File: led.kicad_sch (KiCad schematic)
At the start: 2 parts, among them J6 Conn_01x02

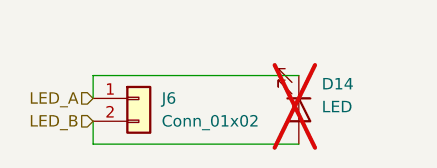
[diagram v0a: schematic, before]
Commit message: board interconnects
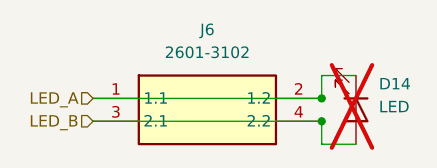
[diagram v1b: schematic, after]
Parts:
- removed J6: Conn_01x02, Connector_Wire:SolderWire-0.75sqmm_1x02_P4.8mm_D1.25mm_OD2.3mm, symbol Connector_Generic:Conn_01x02
- added J6: 2601-3102, KiCad:26013102, symbol 2601-3102:2601-3102
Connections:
- net LED_A: now also J6.1 (1.1), J6.2 (1.2)
- net LED_B: now also J6.3 (2.1), J6.4 (2.2)
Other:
- moved on the sheet: D14
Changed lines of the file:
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@@
 		(comment 3 "Bryan, Tahje")
 	)
-	(wire
-		(pts
-			(xy 171.45 106.68) (xy 148.59 106.68)
-		)
-		(stroke
-			(width 0)
-			(type default)
-		)
-	)
-	(wire
-		(pts
-			(xy 148.59 106.68) (xy 148.59 104.14)
-		)
-		(stroke
-			(width 0)
-			(type default)
-		)
-	)
-	(wire
-		(pts
-			(xy 171.45 99.06) (xy 148.59 99.06)
-		)
-		(stroke
-			(width 0)
-			(type default)
-		)
-	)
-	(wire
-		(pts
-			(xy 148.59 99.06) (xy 148.59 101.6)
+	(junction
+		(at 173.99 104.14)
+		(diameter 0)
+		(color 0 0 0 0)
+	)
+	(junction
+		(at 173.99 101.6)
+		(diameter 0)
+		(color 0 0 0 0)
+	)
+	(wire
+		(pts
+			(xy 148.59 101.6) (xy 173.99 101.6)
+		)
+		(stroke
+			(width 0)
+			(type default)
+		)
+	)
+	(wire
+		(pts
+			(xy 173.99 106.68) (xy 177.8 106.68)
+		)
+		(stroke
+			(width 0)
+			(type default)
+		)
+	)
+	(wire
+		(pts
+			(xy 173.99 104.14) (xy 173.99 106.68)
+		)
+		(stroke
+			(width 0)
+			(type default)
+		)
+	)
+	(wire
+		(pts
+			(xy 148.59 104.14) (xy 173.99 104.14)
+		)
+		(stroke
+			(width 0)
+			(type default)
+		)
+	)
+	(wire
+		(pts
+			(xy 173.99 99.06) (xy 177.8 99.06)
+		)
+		(stroke
+			(width 0)
+			(type default)
+		)
+	)
+	(wire
+		(pts
+			(xy 173.99 101.6) (xy 173.99 99.06)
 		)
 		(stroke
@@
 	(symbol
 		(lib_id "Device:LED")
-		(at 171.45 102.87 270)
+		(at 177.8 102.87 270)
 		(unit 1)
 		(exclude_from_sim no)
@@
 		(dnp yes)
 		(property "Reference" "D14"
-			(at 173.99 100.0124 90)
+			(at 180.34 100.0124 90)
 			(effects
 				(font
@@
 		)
 		(property "Value" "LED"
-			(at 173.99 102.5524 90)
+			(at 180.34 102.5524 90)
 			(effects
 				(font
@@
 		)
 		(property "Footprint" ""
-			(at 171.45 102.87 0)
+			(at 177.8 102.87 0)
 			(effects
 				(font
@@
 		)
 		(property "Datasheet" "https://www.bridgelux.com/sites/default/files/resource_media/DS407%20Gen%208%20V6%20HD%20Array%20Data%20Sheet%2020210520%20Rev%20A.pdf"
-			(at 171.45 102.87 0)
+			(at 177.8 102.87 0)
 			(effects
 				(font
@@
 		)
 		(property "Description" "Light emitting diode"
-			(at 171.45 102.87 0)
+			(at 177.8 102.87 0)
 			(effects
 				(font
@@
 		)
 		(property "Sim.Pins" "1=K 2=A"
-			(at 171.45 102.87 0)
+			(at 177.8 102.87 0)
 			(effects
 				(font
@@
 		)
 		(property "Part Number" "976-BXRH-40H1000-B-83-ND"
-			(at 171.45 102.87 0)
+			(at 177.8 102.87 0)
 			(effects
 				(font
@@
 	)
 	(symbol
-		(lib_id "Connector_Generic:Conn_01x02")
-		(at 153.67 101.6 0)
+		(lib_id "2601-3102:2601-3102")
+		(at 148.59 101.6 0)
 		(unit 1)
 		(exclude_from_sim no)
-		(in_bom no)
+		(in_bom yes)
 		(on_board yes)
 		(dnp no)
 		(fields_autoplaced yes)
 		(property "Reference" "J6"
-			(at 156.21 101.5999 0)
-			(effects
-				(font
-					(size 1.27 1.27)
-				)
-				(justify left)
-			)
-		)
-		(property "Value" "Conn_01x02"
-			(at 156.21 104.1399 0)
-			(effects
-				(font
-					(size 1.27 1.27)
-				)
-				(justify left)
-			)
-		)
-		(property "Footprint" "Connector_Wire:SolderWire-0.75sqmm_1x02_P4.8mm_D1.25mm_OD2.3mm"
-			(at 153.67 101.6 0)
-			(effects
-				(font
-					(size 1.27 1.27)
-				)
-				(hide yes)
-			)
-		)
-		(property "Datasheet" "~"
-			(at 153.67 101.6 0)
-			(effects
-				(font
-					(size 1.27 1.27)
-				)
-				(hide yes)
-			)
-		)
-		(property "Description" "Generic connector, single row, 01x02, script generated (kicad-library-utils/schlib/autogen/connector/)"
-			(at 153.67 101.6 0)
+			(at 161.29 93.98 0)
+			(effects
+				(font
+					(size 1.27 1.27)
+				)
+			)
+		)
+		(property "Value" "2601-3102"
+			(at 161.29 96.52 0)
+			(effects
+				(font
+					(size 1.27 1.27)
+				)
+			)
+		)
+		(property "Footprint" "KiCad:26013102"
+			(at 170.18 196.52 0)
+			(effects
+				(font
+					(size 1.27 1.27)
+				)
+				(justify left top)
+				(hide yes)
+			)
+		)
+		(property "Datasheet" "https://www.wago.com/2601-3102"
+			(at 170.18 296.52 0)
+			(effects
+				(font
+					(size 1.27 1.27)
+				)
+				(justify left top)
+				(hide yes)
+			)
+		)
+		(property "Description" "PCB terminal block; lever; 1.5 mm; Pin spacing 3.5 mm; 2-pole; Push-in CAGE CLAMP"
+			(at 148.59 101.6 0)
+			(effects
+				(font
+					(size 1.27 1.27)
+				)
+				(hide yes)
+			)
+		)
+		(property "Height" "16.58"
+			(at 170.18 496.52 0)
+			(effects
+				(font
+					(size 1.27 1.27)
+				)
+				(justify left top)
+				(hide yes)
+			)
+		)
+		(property "Manufacturer_Name" "Wago"
+			(at 170.18 596.52 0)
+			(effects
+				(font
+					(size 1.27 1.27)
+				)
+				(justify left top)
+				(hide yes)
+			)
+		)
+		(property "Manufacturer_Part_Number" "2601-3102"
+			(at 170.18 696.52 0)
+			(effects
+				(font
+					(size 1.27 1.27)
+				)
+				(justify left top)
+				(hide yes)
+			)
+		)
+		(property "Part Number" "2946-2601-3102-ND"
+			(at 148.59 101.6 0)
 			(effects
 				(font
@@
 		(pin "1"
 		)
+		(pin "3"
+		)
+		(pin "4"
+		)
 		(pin "2"
